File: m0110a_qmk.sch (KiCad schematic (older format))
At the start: 20 parts, among them J1 AVR-ISP-6, J2 USB_B_Mini, Y1 16Mhz

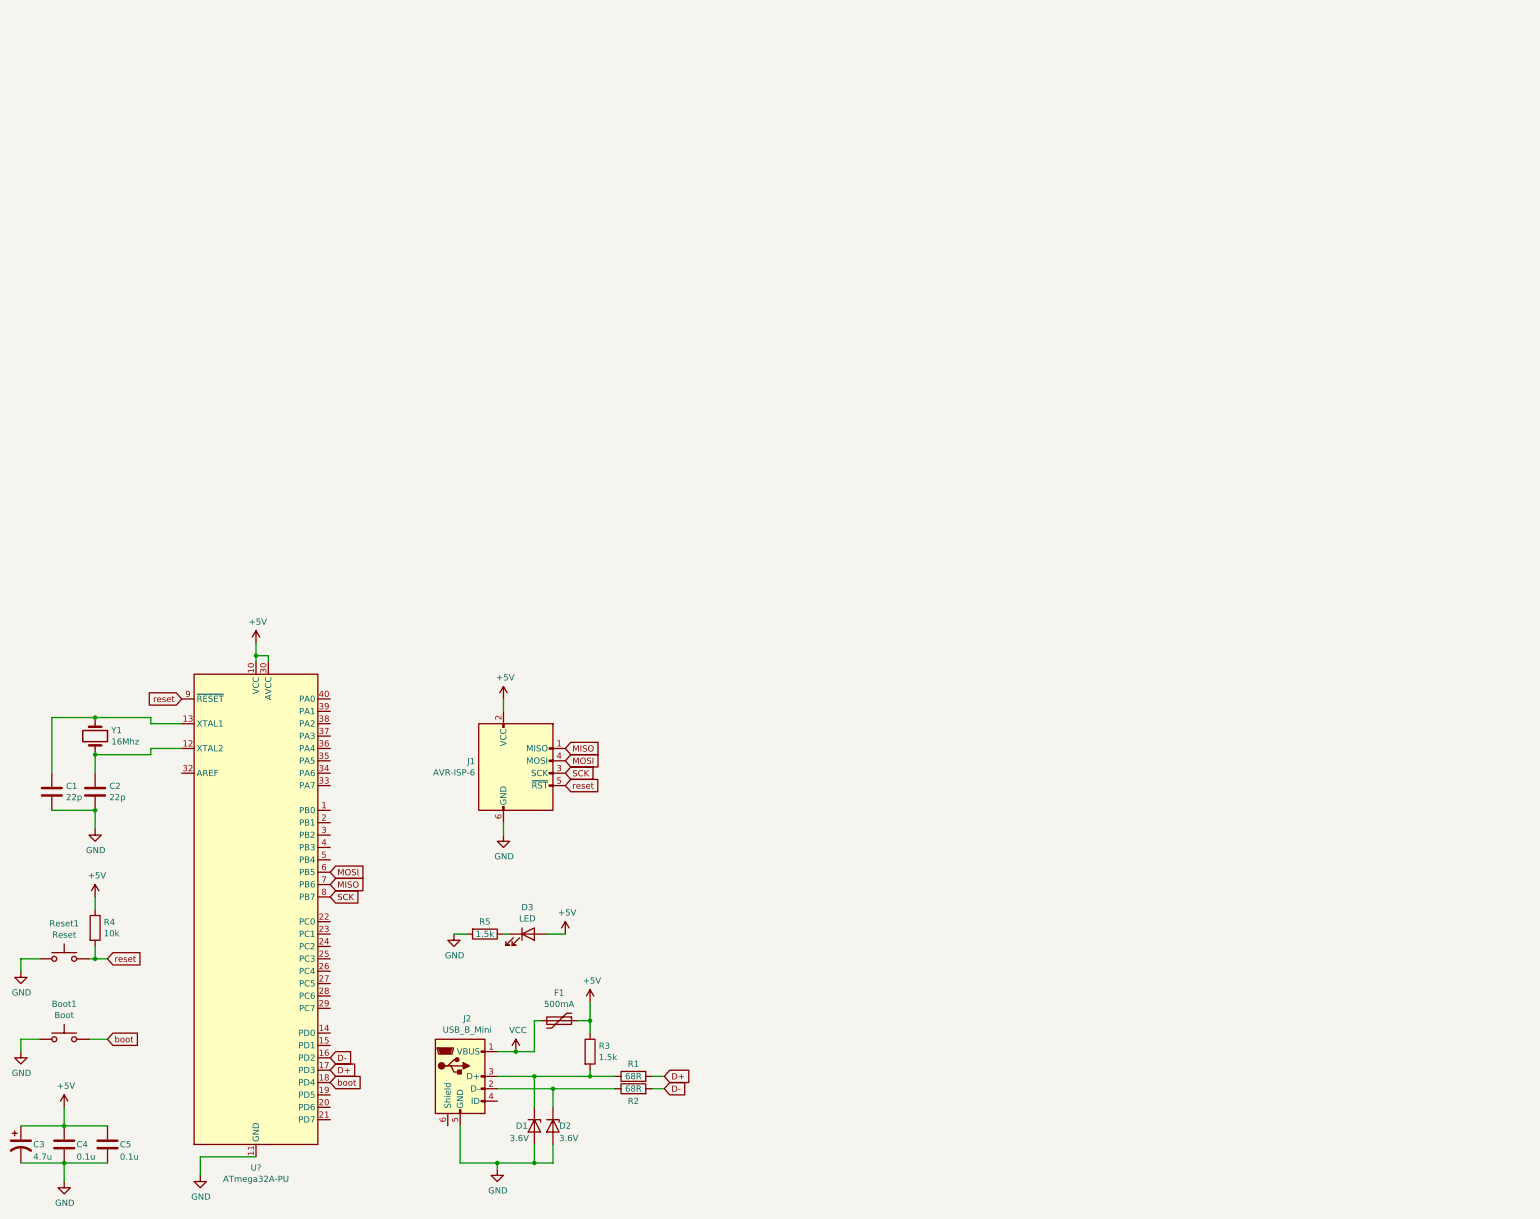
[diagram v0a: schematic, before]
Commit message: finished circuit schema
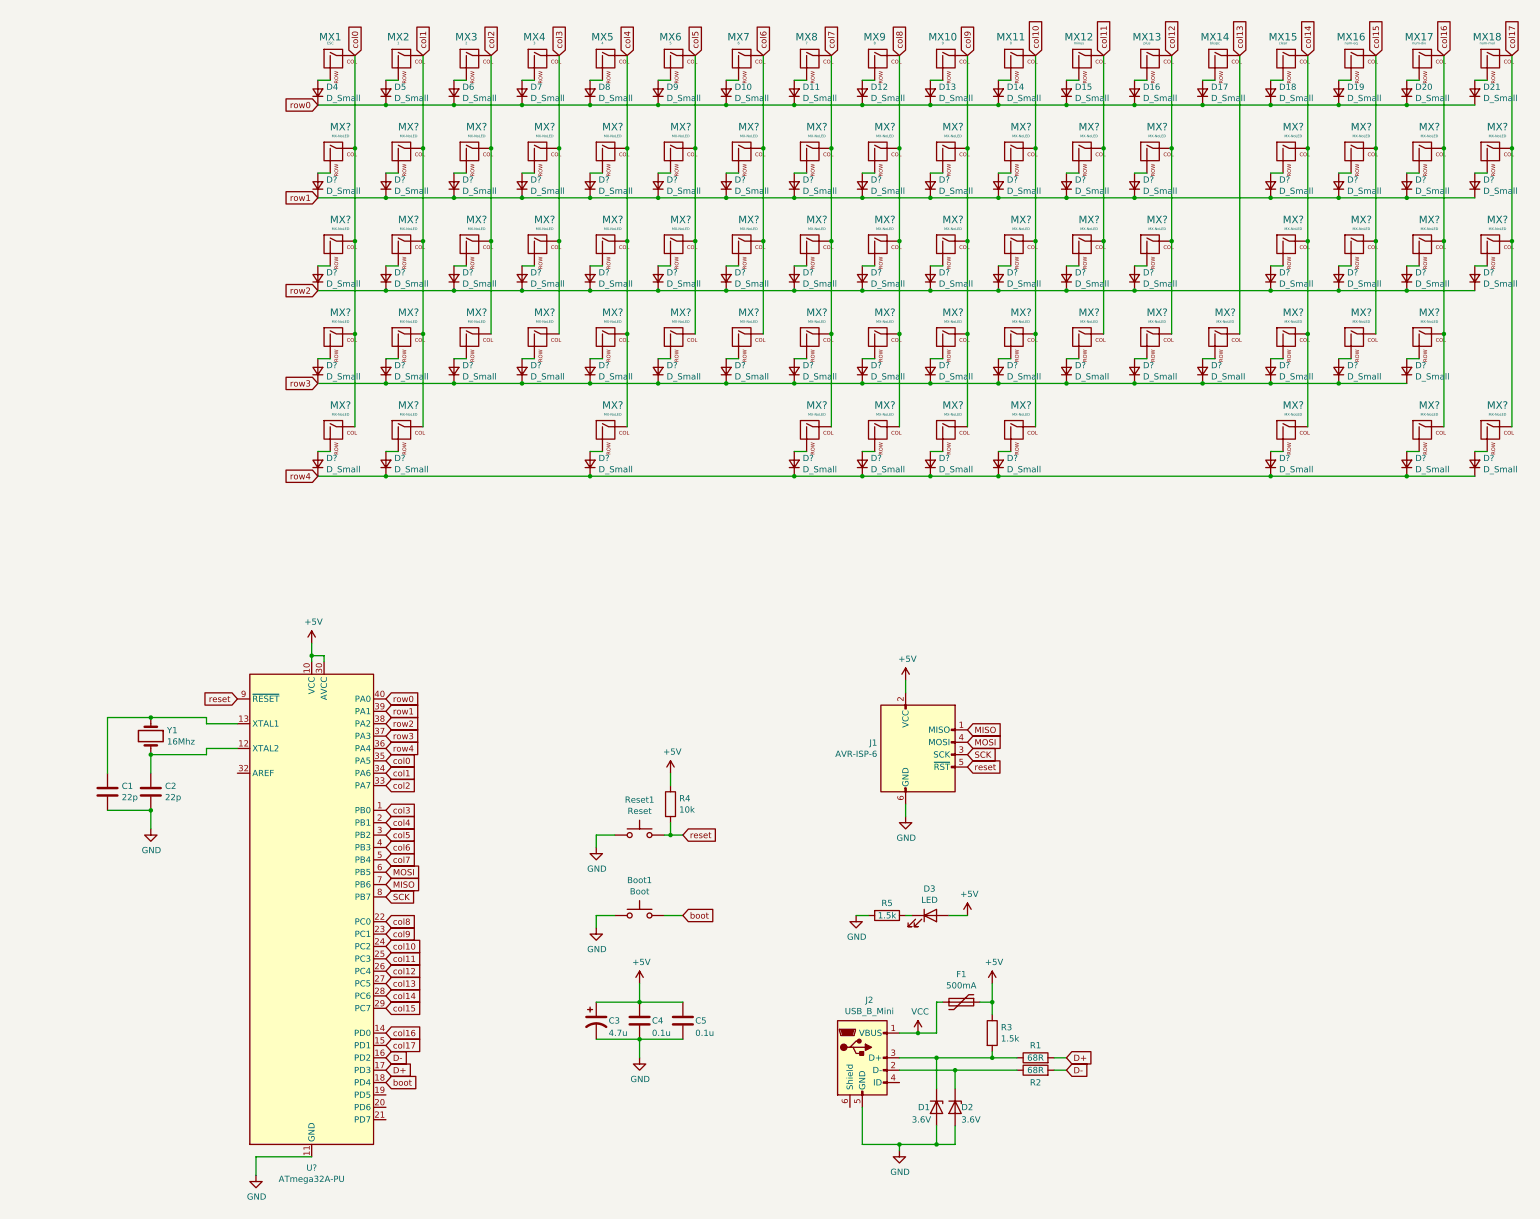
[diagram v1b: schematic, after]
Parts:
- added D10, D11, D12, D13, D14, D15, D16, D17, D18, D19, D20, D21, D4, D5, D6, D7, D8, D9, D? (x61): D_Small, symbol Device:D_Small
- added MX1: ESC, symbol MX_Alps_Hybrid:MX-NoLED
- added MX10: 9, symbol MX_Alps_Hybrid:MX-NoLED
- added MX11: 0, symbol MX_Alps_Hybrid:MX-NoLED
- added MX12: minus, symbol MX_Alps_Hybrid:MX-NoLED
- added MX13: plus, symbol MX_Alps_Hybrid:MX-NoLED
- added MX14: bkspc, symbol MX_Alps_Hybrid:MX-NoLED
- added MX15: clear, symbol MX_Alps_Hybrid:MX-NoLED
- added MX16: num-eq, symbol MX_Alps_Hybrid:MX-NoLED
- added MX17: num-div, symbol MX_Alps_Hybrid:MX-NoLED
- added MX18: num-mul, symbol MX_Alps_Hybrid:MX-NoLED
- added MX2: 1, symbol MX_Alps_Hybrid:MX-NoLED
- added MX3: 2, symbol MX_Alps_Hybrid:MX-NoLED
- added MX4: 3, symbol MX_Alps_Hybrid:MX-NoLED
- added MX5: 4, symbol MX_Alps_Hybrid:MX-NoLED
- added MX6: 5, symbol MX_Alps_Hybrid:MX-NoLED
- added MX7: 6, symbol MX_Alps_Hybrid:MX-NoLED
- added MX8: 7, symbol MX_Alps_Hybrid:MX-NoLED
- added MX9: 8, symbol MX_Alps_Hybrid:MX-NoLED
- added MX? (x61): MX-NoLED, symbol MX_Alps_Hybrid:MX-NoLED
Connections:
- net col3: now reaches U?.1 (PB0)
- net col3: now also MX4.1 (COL), MX?.1 (COL), MX?.1 (COL), MX?.1 (COL)
- net col16: now reaches U?.14 (PD0)
- net col16: now also MX17.1 (COL), MX?.1 (COL), MX?.1 (COL), MX?.1 (COL), MX?.1 (COL)
- net col17: now reaches U?.15 (PD1)
- net col17: now also MX18.1 (COL), MX?.1 (COL), MX?.1 (COL), MX?.1 (COL)
- net col4: now reaches U?.2 (PB1)
- net col4: now also MX5.1 (COL), MX?.1 (COL), MX?.1 (COL), MX?.1 (COL), MX?.1 (COL)
- net col8: now reaches U?.22 (PC0)
- net col8: now also MX9.1 (COL), MX?.1 (COL), MX?.1 (COL), MX?.1 (COL), MX?.1 (COL)
- net col9: now reaches U?.23 (PC1)
- net col9: now also MX10.1 (COL), MX?.1 (COL), MX?.1 (COL), MX?.1 (COL), MX?.1 (COL)
- net col10: now reaches U?.24 (PC2)
- net col10: now also MX11.1 (COL), MX?.1 (COL), MX?.1 (COL), MX?.1 (COL), MX?.1 (COL)
- net col11: now reaches U?.25 (PC3)
- net col11: now also MX12.1 (COL), MX?.1 (COL), MX?.1 (COL), MX?.1 (COL)
- net col12: now reaches U?.26 (PC4)
- net col12: now also MX13.1 (COL), MX?.1 (COL), MX?.1 (COL), MX?.1 (COL)
- net col13: now reaches U?.27 (PC5)
- net col13: now also MX14.1 (COL), MX?.1 (COL)
- net col14: now reaches U?.28 (PC6)
- net col14: now also MX15.1 (COL), MX?.1 (COL), MX?.1 (COL), MX?.1 (COL), MX?.1 (COL)
- net col15: now reaches U?.29 (PC7)
- net col15: now also MX16.1 (COL), MX?.1 (COL), MX?.1 (COL), MX?.1 (COL)
- net col5: now reaches U?.3 (PB2)
- net col5: now also MX6.1 (COL), MX?.1 (COL), MX?.1 (COL), MX?.1 (COL)
- net col2: now reaches U?.33 (PA7)
- net col2: now also MX3.1 (COL), MX?.1 (COL), MX?.1 (COL), MX?.1 (COL)
- net col1: now reaches U?.34 (PA6)
- net col1: now also MX2.1 (COL), MX?.1 (COL), MX?.1 (COL), MX?.1 (COL), MX?.1 (COL)
- net col0: now reaches U?.35 (PA5)
- net col0: now also MX1.1 (COL), MX?.1 (COL), MX?.1 (COL), MX?.1 (COL), MX?.1 (COL)
- net row4: now reaches U?.36 (PA4)
- net row4: now also D?.1 (K), D?.1 (K), D?.1 (K), D?.1 (K), D?.1 (K), D?.1 (K), D?.1 (K), D?.1 (K), D?.1 (K), D?.1 (K)
- net row3: now reaches U?.37 (PA3)
- net row3: now also D?.1 (K), D?.1 (K), D?.1 (K), D?.1 (K), D?.1 (K), D?.1 (K), D?.1 (K), D?.1 (K), D?.1 (K), D?.1 (K), D?.1 (K), D?.1 (K), D?.1 (K), D?.1 (K), D?.1 (K), D?.1 (K), D?.1 (K)
- net row2: now reaches U?.38 (PA2)
- net row2: now also D?.1 (K), D?.1 (K), D?.1 (K), D?.1 (K), D?.1 (K), D?.1 (K), D?.1 (K), D?.1 (K), D?.1 (K), D?.1 (K), D?.1 (K), D?.1 (K), D?.1 (K), D?.1 (K), D?.1 (K), D?.1 (K), D?.1 (K)
- net row1: now reaches U?.39 (PA1)
- net row1: now also D?.1 (K), D?.1 (K), D?.1 (K), D?.1 (K), D?.1 (K), D?.1 (K), D?.1 (K), D?.1 (K), D?.1 (K), D?.1 (K), D?.1 (K), D?.1 (K), D?.1 (K), D?.1 (K), D?.1 (K), D?.1 (K), D?.1 (K)
- net col6: now reaches U?.4 (PB3)
- net col6: now also MX7.1 (COL), MX?.1 (COL), MX?.1 (COL), MX?.1 (COL)
- net row0: now reaches U?.40 (PA0)
- net row0: now also D10.1 (K), D11.1 (K), D12.1 (K), D13.1 (K), D14.1 (K), D15.1 (K), D16.1 (K), D17.1 (K), D18.1 (K), D19.1 (K), D20.1 (K), D21.1 (K), D4.1 (K), D5.1 (K), D6.1 (K), D7.1 (K), D8.1 (K), D9.1 (K)
- net col7: now reaches U?.5 (PB4)
- net col7: now also MX8.1 (COL), MX?.1 (COL), MX?.1 (COL), MX?.1 (COL), MX?.1 (COL)
- new net: D4.2 (A), MX1.2 (ROW)
- new net: D5.2 (A), MX2.2 (ROW)
- new net: D6.2 (A), MX3.2 (ROW)
- new net: D7.2 (A), MX4.2 (ROW)
- new net: D8.2 (A), MX5.2 (ROW)
- new net: D9.2 (A), MX6.2 (ROW)
- new net: D10.2 (A), MX7.2 (ROW)
- new net: D11.2 (A), MX8.2 (ROW)
- new net: D12.2 (A), MX9.2 (ROW)
- new net: D13.2 (A), MX10.2 (ROW)
- new net: D14.2 (A), MX11.2 (ROW)
- new net: D15.2 (A), MX12.2 (ROW)
- new net: D16.2 (A), MX13.2 (ROW)
- new net: D17.2 (A), MX14.2 (ROW)
- new net: D18.2 (A), MX15.2 (ROW)
- new net: D19.2 (A), MX16.2 (ROW)
- new net: D20.2 (A), MX17.2 (ROW)
- new net: D21.2 (A), MX18.2 (ROW)
- new net: D?.2 (A), MX?.2 (ROW) (x61)
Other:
- moved on the sheet: Boot1, C1, C2, C3, C4, C5, D1, D2, D3, F1, J1, J2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
